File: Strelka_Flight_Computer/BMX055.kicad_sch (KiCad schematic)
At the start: 3 parts, among them U11 BMX055

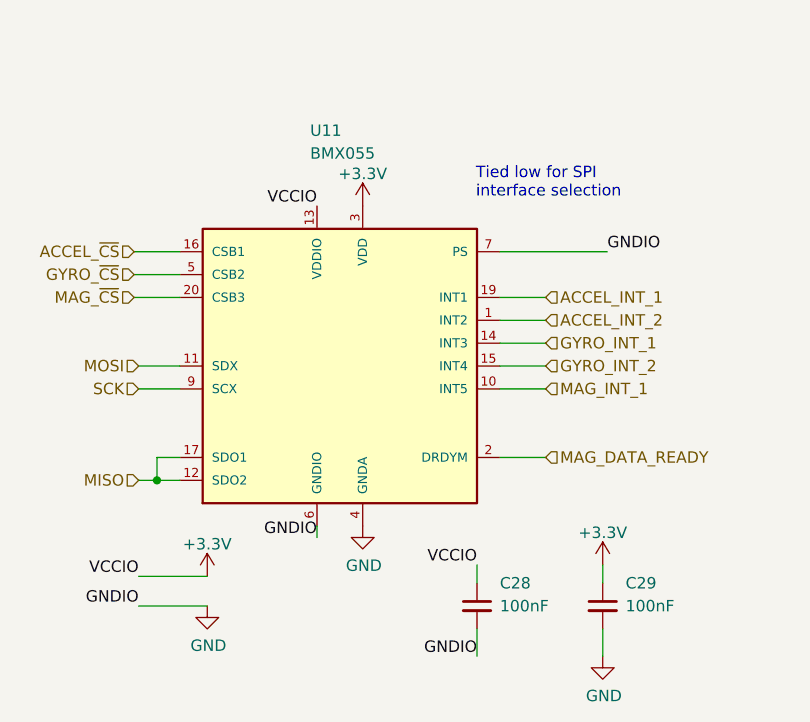
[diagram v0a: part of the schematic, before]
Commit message: Continued routing
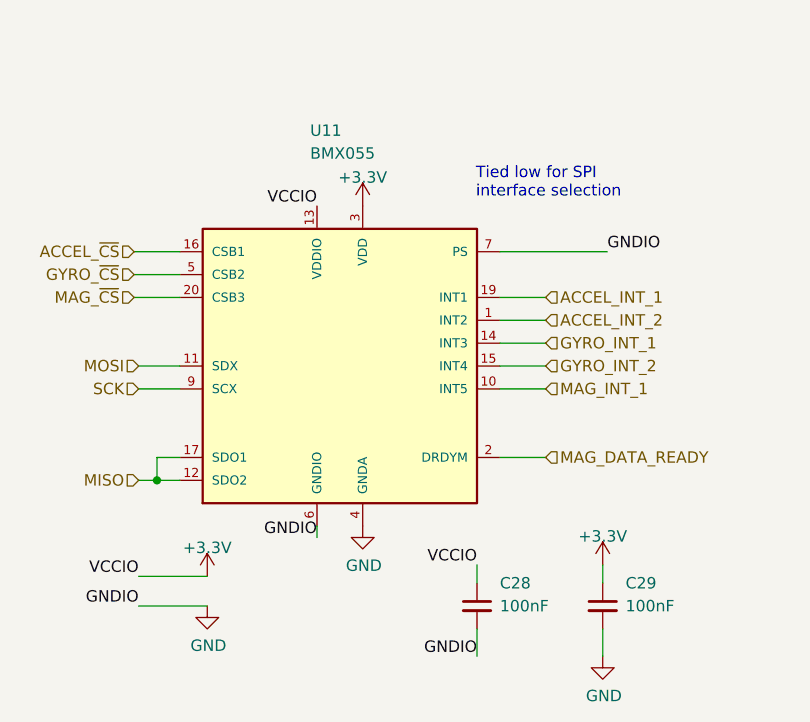
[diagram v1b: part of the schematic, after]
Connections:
- net +3V3 renamed +3.3V
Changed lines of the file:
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@@
     (effects (font (size 1.27 1.27)) (justify left))
   )
-  (symbol (lib_id "power:+3.3V") (at 153.162 75.692 0) (unit 1)
+  (symbol (lib_id "power:GND") (at 179.832 125.73 0) (unit 1)
+    (in_bom yes) (on_board yes) (dnp no)
+    (property "Reference" "#PWR0176" (at 179.832 132.08 0)
+      (effects (font (size 1.27 1.27)) hide)
+    )
+    (property "Value" "GND" (at 179.959 130.1242 0)
+      (effects (font (size 1.27 1.27)))
+    )
+    (property "Footprint" "" (at 179.832 125.73 0)
+      (effects (font (size 1.27 1.27)) hide)
+    )
+    (property "Datasheet" "" (at 179.832 125.73 0)
+      (effects (font (size 1.27 1.27)) hide)
+    )
+    (pin "1")
+    (instances
+      (project "Strelka_Flight_Computer"
+        (path "/e63e39d7-6ac0-4ffd-8aa3-1841a4541b55/78f71895-bddb-4f64-a608-99074f2d1c44/256d0f41-abcb-432e-a4cc-bcef1aa15bc3"
+          (reference "#PWR0176") (unit 1)
+        )
+      )
+    )
+  )
+  (symbol (lib_name "+3.3V_1") (lib_id "power:+3.3V") (at 179.832 115.57 0) (unit 1)
     (in_bom yes) (on_board yes) (dnp no) (fields_autoplaced)
-    (property "Reference" "#PWR0172" (at 153.162 79.502 0)
-      (effects (font (size 1.27 1.27)) hide)
-    )
-    (property "Value" "+3.3V" (at 153.162 72.1162 0)
-      (effects (font (size 1.27 1.27)))
-    )
-    (property "Footprint" "" (at 153.162 75.692 0)
-      (effects (font (size 1.27 1.27)) hide)
-    )
-    (property "Datasheet" "" (at 153.162 75.692 0)
-      (effects (font (size 1.27 1.27)) hide)
-    )
-    (pin "1")
-    (instances
-      (project "Strelka_Flight_Computer"
-        (path "/e63e39d7-6ac0-4ffd-8aa3-1841a4541b55/78f71895-bddb-4f64-a608-99074f2d1c44/256d0f41-abcb-432e-a4cc-bcef1aa15bc3"
-          (reference "#PWR0172") (unit 1)
-        )
-      )
-    )
-  )
-  (symbol (lib_id "power:GND") (at 179.832 125.73 0) (unit 1)
-    (in_bom yes) (on_board yes) (dnp no)
-    (property "Reference" "#PWR0176" (at 179.832 132.08 0)
-      (effects (font (size 1.27 1.27)) hide)
-    )
-    (property "Value" "GND" (at 179.959 130.1242 0)
-      (effects (font (size 1.27 1.27)))
-    )
-    (property "Footprint" "" (at 179.832 125.73 0)
-      (effects (font (size 1.27 1.27)) hide)
-    )
-    (property "Datasheet" "" (at 179.832 125.73 0)
-      (effects (font (size 1.27 1.27)) hide)
-    )
-    (pin "1")
-    (instances
-      (project "Strelka_Flight_Computer"
-        (path "/e63e39d7-6ac0-4ffd-8aa3-1841a4541b55/78f71895-bddb-4f64-a608-99074f2d1c44/256d0f41-abcb-432e-a4cc-bcef1aa15bc3"
-          (reference "#PWR0176") (unit 1)
+    (property "Reference" "#PWR07" (at 179.832 119.38 0)
+      (effects (font (size 1.27 1.27)) hide)
+    )
+    (property "Value" "+3.3V" (at 179.832 112.395 0)
+      (effects (font (size 1.27 1.27)))
+    )
+    (property "Footprint" "" (at 179.832 115.57 0)
+      (effects (font (size 1.27 1.27)) hide)
+    )
+    (property "Datasheet" "" (at 179.832 115.57 0)
+      (effects (font (size 1.27 1.27)) hide)
+    )
+    (pin "1")
+    (instances
+      (project "Strelka_Flight_Computer"
+        (path "/e63e39d7-6ac0-4ffd-8aa3-1841a4541b55/e94c6cea-6c6c-4b5f-a840-b97a15d9406a"
+          (reference "#PWR07") (unit 1)
+        )
+        (path "/e63e39d7-6ac0-4ffd-8aa3-1841a4541b55/78f71895-bddb-4f64-a608-99074f2d1c44/256d0f41-abcb-432e-a4cc-bcef1aa15bc3"
+          (reference "#PWR012") (unit 1)
         )
       )
@@
     )
   )
-  (symbol (lib_id "power:+3.3V") (at 179.832 115.57 0) (unit 1)
+  (symbol (lib_name "+3.3V_1") (lib_id "power:+3.3V") (at 153.162 75.692 0) (unit 1)
     (in_bom yes) (on_board yes) (dnp no) (fields_autoplaced)
-    (property "Reference" "#PWR0177" (at 179.832 119.38 0)
-      (effects (font (size 1.27 1.27)) hide)
-    )
-    (property "Value" "+3.3V" (at 179.832 111.9942 0)
-      (effects (font (size 1.27 1.27)))
-    )
-    (property "Footprint" "" (at 179.832 115.57 0)
-      (effects (font (size 1.27 1.27)) hide)
-    )
-    (property "Datasheet" "" (at 179.832 115.57 0)
-      (effects (font (size 1.27 1.27)) hide)
-    )
-    (pin "1")
-    (instances
-      (project "Strelka_Flight_Computer"
-        (path "/e63e39d7-6ac0-4ffd-8aa3-1841a4541b55/78f71895-bddb-4f64-a608-99074f2d1c44/256d0f41-abcb-432e-a4cc-bcef1aa15bc3"
-          (reference "#PWR0177") (unit 1)
-        )
-      )
-    )
-  )
-  (symbol (lib_id "power:+3.3V") (at 135.89 116.84 0) (unit 1)
+    (property "Reference" "#PWR07" (at 153.162 79.502 0)
+      (effects (font (size 1.27 1.27)) hide)
+    )
+    (property "Value" "+3.3V" (at 153.162 72.517 0)
+      (effects (font (size 1.27 1.27)))
+    )
+    (property "Footprint" "" (at 153.162 75.692 0)
+      (effects (font (size 1.27 1.27)) hide)
+    )
+    (property "Datasheet" "" (at 153.162 75.692 0)
+      (effects (font (size 1.27 1.27)) hide)
+    )
+    (pin "1")
+    (instances
+      (project "Strelka_Flight_Computer"
+        (path "/e63e39d7-6ac0-4ffd-8aa3-1841a4541b55/e94c6cea-6c6c-4b5f-a840-b97a15d9406a"
+          (reference "#PWR07") (unit 1)
+        )
+        (path "/e63e39d7-6ac0-4ffd-8aa3-1841a4541b55/78f71895-bddb-4f64-a608-99074f2d1c44/256d0f41-abcb-432e-a4cc-bcef1aa15bc3"
+          (reference "#PWR013") (unit 1)
+        )
+      )
+    )
+  )
+  (symbol (lib_name "+3.3V_1") (lib_id "power:+3.3V") (at 135.89 116.84 0) (unit 1)
     (in_bom yes) (on_board yes) (dnp no) (fields_autoplaced)
-    (property "Reference" "#PWR0175" (at 135.89 120.65 0)
-      (effects (font (size 1.27 1.27)) hide)
-    )
-    (property "Value" "+3.3V" (at 135.89 113.2642 0)
+    (property "Reference" "#PWR07" (at 135.89 120.65 0)
+      (effects (font (size 1.27 1.27)) hide)
+    )
+    (property "Value" "+3.3V" (at 135.89 113.665 0)
       (effects (font (size 1.27 1.27)))
     )
@@
     (instances
       (project "Strelka_Flight_Computer"
-        (path "/e63e39d7-6ac0-4ffd-8aa3-1841a4541b55/78f71895-bddb-4f64-a608-99074f2d1c44/256d0f41-abcb-432e-a4cc-bcef1aa15bc3"
-          (reference "#PWR0175") (unit 1)
-        )
-      )
+        (path "/e63e39d7-6ac0-4ffd-8aa3-1841a4541b55/e94c6cea-6c6c-4b5f-a840-b97a15d9406a"
+          (reference "#PWR07") (unit 1)
+        )
+        (path "/e63e39d7-6ac0-4ffd-8aa3-1841a4541b55/78f71895-bddb-4f64-a608-99074f2d1c44/256d0f41-abcb-432e-a4cc-bcef1aa15bc3"
+          (reference "#PWR011") (unit 1)
+        )
+      )
